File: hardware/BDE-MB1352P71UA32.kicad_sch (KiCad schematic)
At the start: 11 parts, among them J401 Conn_ARM_JTAG_SWD_10, SW401 SW_Push, U401 BDE-MB1352P71UA32, U402 USBLC6-2P6, U403 USBLC6-2P6

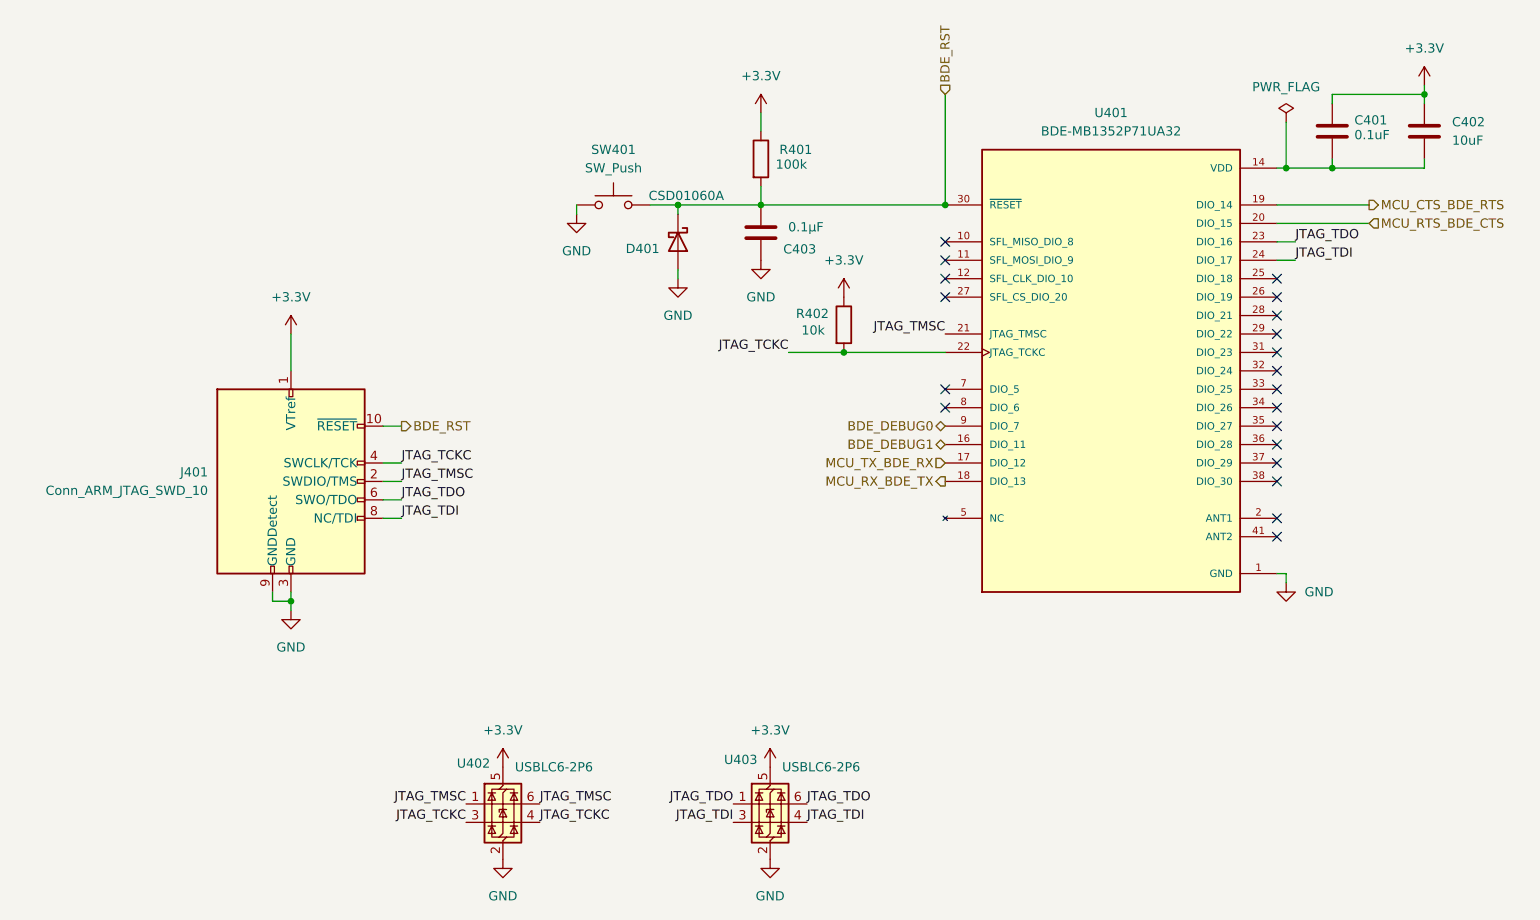
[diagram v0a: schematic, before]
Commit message: reannotate
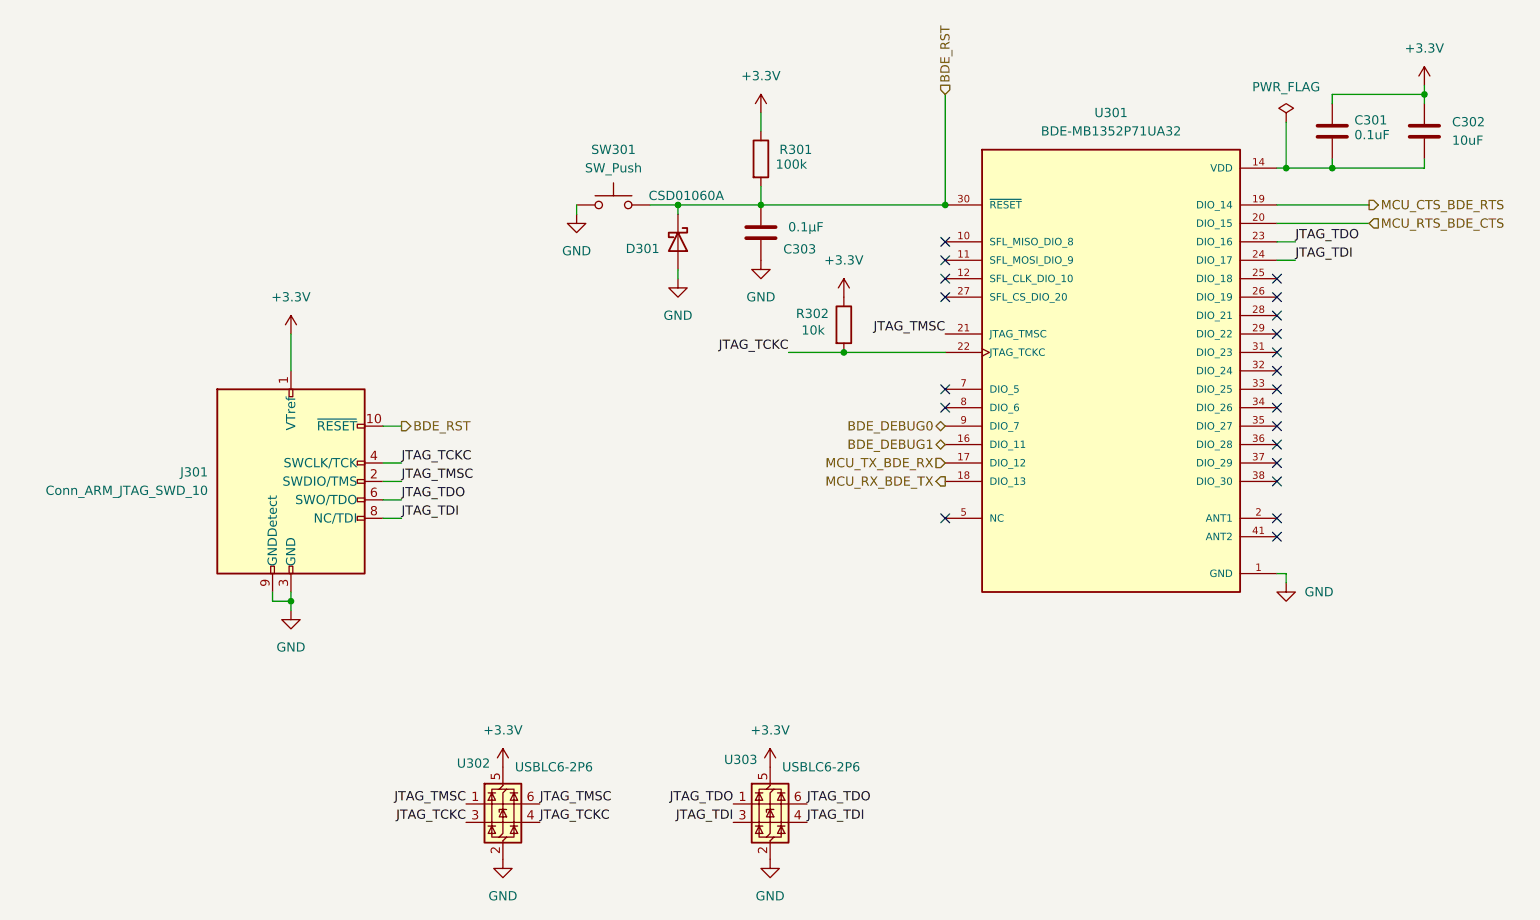
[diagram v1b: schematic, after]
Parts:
- renumbered C401 to C301, C402 to C302, C403 to C303, D401 to D301, J401 to J301, R401 to R301, R402 to R302, SW401 to SW301, U401 to U301, U402 to U302, U403 to U303
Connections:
- no-connect marks 20 -> 21
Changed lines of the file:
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@@
+	)
+	(no_connect
+		(at 166.37 105.41)
 	)
 	(no_connect
@@
 		(dnp no)
 		(fields_autoplaced yes)
-		(property "Reference" "#PWR0411"
+		(property "Reference" "#PWR0311"
 			(at 142.24 143.51 0)
 			(effects
@@
 			(project "Senior_Design"
 				(path "/8f5928e8-0fc1-4443-a20f-3bfeb956761e/dd2813e4-a810-44d7-8b7e-d46ce1c3fa30"
-					(reference "#PWR0411")
+					(reference "#PWR0311")
 					(unit 1)
 				)
@@
 		(dnp no)
 		(fields_autoplaced yes)
-		(property "Reference" "#PWR0406"
+		(property "Reference" "#PWR0306"
 			(at 152.4 78.74 0)
 			(effects
@@
 			(project "Senior_Design"
 				(path "/8f5928e8-0fc1-4443-a20f-3bfeb956761e/dd2813e4-a810-44d7-8b7e-d46ce1c3fa30"
-					(reference "#PWR0406")
+					(reference "#PWR0306")
 					(unit 1)
 				)
@@
 		(on_board yes)
 		(dnp no)
-		(property "Reference" "U403"
+		(property "Reference" "U303"
 			(at 135.89 138.684 0)
 			(effects
@@
 			(project "Senior_Design"
 				(path "/8f5928e8-0fc1-4443-a20f-3bfeb956761e/dd2813e4-a810-44d7-8b7e-d46ce1c3fa30"
-					(reference "U403")
+					(reference "U303")
 					(unit 1)
 				)
@@
 		(dnp no)
 		(fields_autoplaced yes)
-		(property "Reference" "#PWR0405"
+		(property "Reference" "#PWR0305"
 			(at 129.54 78.74 0)
 			(effects
@@
 			(project "Senior_Design"
 				(path "/8f5928e8-0fc1-4443-a20f-3bfeb956761e/dd2813e4-a810-44d7-8b7e-d46ce1c3fa30"
-					(reference "#PWR0405")
+					(reference "#PWR0305")
 					(unit 1)
 				)
@@
 		(on_board yes)
 		(dnp no)
-		(property "Reference" "C401"
+		(property "Reference" "C301"
 			(at 222.758 50.546 0)
 			(effects
@@
 			(project "Senior_Design"
 				(path "/8f5928e8-0fc1-4443-a20f-3bfeb956761e/dd2813e4-a810-44d7-8b7e-d46ce1c3fa30"
-					(reference "C401")
+					(reference "C301")
 					(unit 1)
 				)
@@
 		(dnp no)
 		(fields_autoplaced yes)
-		(property "Reference" "J401"
+		(property "Reference" "J301"
 			(at 64.77 99.0599 0)
 			(effects
@@
 			(project "Senior_Design"
 				(path "/8f5928e8-0fc1-4443-a20f-3bfeb956761e/dd2813e4-a810-44d7-8b7e-d46ce1c3fa30"
-					(reference "J401")
+					(reference "J301")
 					(unit 1)
 				)
@@
 		(on_board yes)
 		(dnp no)
-		(property "Reference" "U402"
+		(property "Reference" "U302"
 			(at 99.06 139.192 0)
 			(effects
@@
 			(project "Senior_Design"
 				(path "/8f5928e8-0fc1-4443-a20f-3bfeb956761e/dd2813e4-a810-44d7-8b7e-d46ce1c3fa30"
-					(reference "U402")
+					(reference "U302")
 					(unit 1)
 				)
@@
 		(dnp no)
 		(fields_autoplaced yes)
-		(property "Reference" "#PWR0409"
+		(property "Reference" "#PWR0309"
 			(at 76.2 124.46 0)
 			(effects
@@
 			(project "Senior_Design"
 				(path "/8f5928e8-0fc1-4443-a20f-3bfeb956761e/dd2813e4-a810-44d7-8b7e-d46ce1c3fa30"
-					(reference "#PWR0409")
+					(reference "#PWR0309")
 					(unit 1)
 				)
@@
 		(on_board yes)
 		(dnp no)
-		(property "Reference" "C403"
+		(property "Reference" "C303"
 			(at 148.59 68.326 0)
 			(effects
@@
 			(project "Senior_Design"
 				(path "/8f5928e8-0fc1-4443-a20f-3bfeb956761e/dd2813e4-a810-44d7-8b7e-d46ce1c3fa30"
-					(reference "C403")
+					(reference "C303")
 					(unit 1)
 				)
@@
 		(dnp no)
 		(fields_autoplaced yes)
-		(property "Reference" "#PWR0404"
+		(property "Reference" "#PWR0304"
 			(at 140.97 76.2 0)
 			(effects
@@
 			(project "Senior_Design"
 				(path "/8f5928e8-0fc1-4443-a20f-3bfeb956761e/dd2813e4-a810-44d7-8b7e-d46ce1c3fa30"
-					(reference "#PWR0404")
+					(reference "#PWR0304")
 					(unit 1)
 				)
@@
 		(dnp no)
 		(fields_autoplaced yes)
-		(property "Reference" "#PWR0410"
+		(property "Reference" "#PWR0310"
 			(at 105.41 143.51 0)
 			(effects
@@
 			(project "Senior_Design"
 				(path "/8f5928e8-0fc1-4443-a20f-3bfeb956761e/dd2813e4-a810-44d7-8b7e-d46ce1c3fa30"
-					(reference "#PWR0410")
+					(reference "#PWR0310")
 					(unit 1)
 				)
@@
 		(dnp no)
 		(fields_autoplaced yes)
-		(property "Reference" "U401"
+		(property "Reference" "U301"
 			(at 189.23 49.53 0)
 			(effects
@@
 			(project "Senior_Design"
 				(path "/8f5928e8-0fc1-4443-a20f-3bfeb956761e/dd2813e4-a810-44d7-8b7e-d46ce1c3fa30"
-					(reference "U401")
+					(reference "U301")
 					(unit 1)
 				)
@@
 		(dnp no)
 		(fields_autoplaced yes)
-		(property "Reference" "#PWR0402"
+		(property "Reference" "#PWR0302"
 			(at 140.97 53.34 0)
 			(effects
@@
 			(project "Senior_Design"
 				(path "/8f5928e8-0fc1-4443-a20f-3bfeb956761e/dd2813e4-a810-44d7-8b7e-d46ce1c3fa30"
-					(reference "#PWR0402")
+					(reference "#PWR0302")
 					(unit 1)
 				)
@@
 		(dnp no)
 		(fields_autoplaced yes)
-		(property "Reference" "SW401"
+		(property "Reference" "SW301"
 			(at 120.65 54.61 0)
 			(effects
@@
 			(project "Senior_Design"
 				(path "/8f5928e8-0fc1-4443-a20f-3bfeb956761e/dd2813e4-a810-44d7-8b7e-d46ce1c3fa30"
-					(reference "SW401")
+					(reference "SW301")
 					(unit 1)
 				)
@@
 		(dnp no)
 		(fields_autoplaced yes)
-		(property "Reference" "#PWR0407"
+		(property "Reference" "#PWR0307"
 			(at 76.2 83.82 0)
 			(effects
@@
 			(project "Senior_Design"
 				(path "/8f5928e8-0fc1-4443-a20f-3bfeb956761e/dd2813e4-a810-44d7-8b7e-d46ce1c3fa30"
-					(reference "#PWR0407")
+					(reference "#PWR0307")
 					(unit 1)
 				)
@@
 		(on_board yes)
 		(dnp no)
-		(property "Reference" "D401"
+		(property "Reference" "D301"
 			(at 127 68.2626 90)
 			(effects
@@
 			(project "Senior_Design"
 				(path "/8f5928e8-0fc1-4443-a20f-3bfeb956761e/dd2813e4-a810-44d7-8b7e-d46ce1c3fa30"
-					(reference "D401")
+					(reference "D301")
 					(unit 1)
 				)
@@
 		(dnp no)
 		(fields_autoplaced yes)
-		(property "Reference" "#PWR0408"
+		(property "Reference" "#PWR0308"
 			(at 213.36 120.65 0)
 			(effects
@@
 			(project "Senior_Design"
 				(path "/8f5928e8-0fc1-4443-a20f-3bfeb956761e/dd2813e4-a810-44d7-8b7e-d46ce1c3fa30"
-					(reference "#PWR0408")
+					(reference "#PWR0308")
 					(unit 1)
 				)
@@
 		(dnp no)
 		(fields_autoplaced yes)
-		(property "Reference" "#PWR0403"
+		(property "Reference" "#PWR0303"
 			(at 115.57 69.85 0)
 			(effects
@@
 			(project "Senior_Design"
 				(path "/8f5928e8-0fc1-4443-a20f-3bfeb956761e/dd2813e4-a810-44d7-8b7e-d46ce1c3fa30"
-					(reference "#PWR0403")
+					(reference "#PWR0303")
 					(unit 1)
 				)
@@
 		(dnp no)
 		(fields_autoplaced yes)
-		(property "Reference" "C402"
+		(property "Reference" "C302"
 			(at 236.22 50.7999 0)
 			(effects
@@
 			(project "Senior_Design"
 				(path "/8f5928e8-0fc1-4443-a20f-3bfeb956761e/dd2813e4-a810-44d7-8b7e-d46ce1c3fa30"
-					(reference "C402")
+					(reference "C302")
 					(unit 1)
 				)
@@
 		(dnp no)
 		(fields_autoplaced yes)
-		(property "Reference" "#PWR0412"
+		(property "Reference" "#PWR0312"
 			(at 105.41 158.75 0)
 			(effects
@@
 			(project "Senior_Design"
 				(path "/8f5928e8-0fc1-4443-a20f-3bfeb956761e/dd2813e4-a810-44d7-8b7e-d46ce1c3fa30"
-					(reference "#PWR0412")
+					(reference "#PWR0312")
 					(unit 1)
 				)
@@
 		(on_board yes)
 		(dnp no)
-		(property "Reference" "R401"
+		(property "Reference" "R301"
 			(at 143.51 54.6099 0)
 			(effects
@@
 			(project "Senior_Design"
 				(path "/8f5928e8-0fc1-4443-a20f-3bfeb956761e/dd2813e4-a810-44d7-8b7e-d46ce1c3fa30"
-					(reference "R401")
+					(reference "R301")
 					(unit 1)
 				)
@@
 		(dnp no)
 		(fields_autoplaced yes)
-		(property "Reference" "#PWR0413"
+		(property "Reference" "#PWR0313"
 			(at 142.24 158.75 0)
 			(effects
@@
 			(project "Senior_Design"
 				(path "/8f5928e8-0fc1-4443-a20f-3bfeb956761e/dd2813e4-a810-44d7-8b7e-d46ce1c3fa30"
-					(reference "#PWR0413")
+					(reference "#PWR0313")
 					(unit 1)
 				)
@@
 		(on_board yes)
 		(dnp no)
-		(property "Reference" "R402"
+		(property "Reference" "R302"
 			(at 145.796 77.216 0)
 			(effects
@@
 			(project "Senior_Design"
 				(path "/8f5928e8-0fc1-4443-a20f-3bfeb956761e/dd2813e4-a810-44d7-8b7e-d46ce1c3fa30"
-					(reference "R402")
+					(reference "R302")
 					(unit 1)
 				)
@@
 		(on_board yes)
 		(dnp no)
-		(property "Reference" "#FLG0401"
+		(property "Reference" "#FLG0301"
 			(at 213.36 48.895 0)
 			(effects
@@
 			(project "Senior_Design"
 				(path "/8f5928e8-0fc1-4443-a20f-3bfeb956761e/dd2813e4-a810-44d7-8b7e-d46ce1c3fa30"
-					(reference "#FLG0401")
+					(reference "#FLG0301")
 					(unit 1)
 				)
@@
 		(dnp no)
 		(fields_autoplaced yes)
-		(property "Reference" "#PWR0401"
+		(property "Reference" "#PWR0301"
 			(at 232.41 49.53 0)
 			(effects
@@
 			(project "Senior_Design"
 				(path "/8f5928e8-0fc1-4443-a20f-3bfeb956761e/dd2813e4-a810-44d7-8b7e-d46ce1c3fa30"
-					(reference "#PWR0401")
+					(reference "#PWR0301")
 					(unit 1)
 				)
